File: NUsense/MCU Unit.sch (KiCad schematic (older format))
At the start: 45 parts, among them SW301 SW_Push, U301 STM32F746ZGT6, X301 24MHz, X302 ST3215SB32768H5

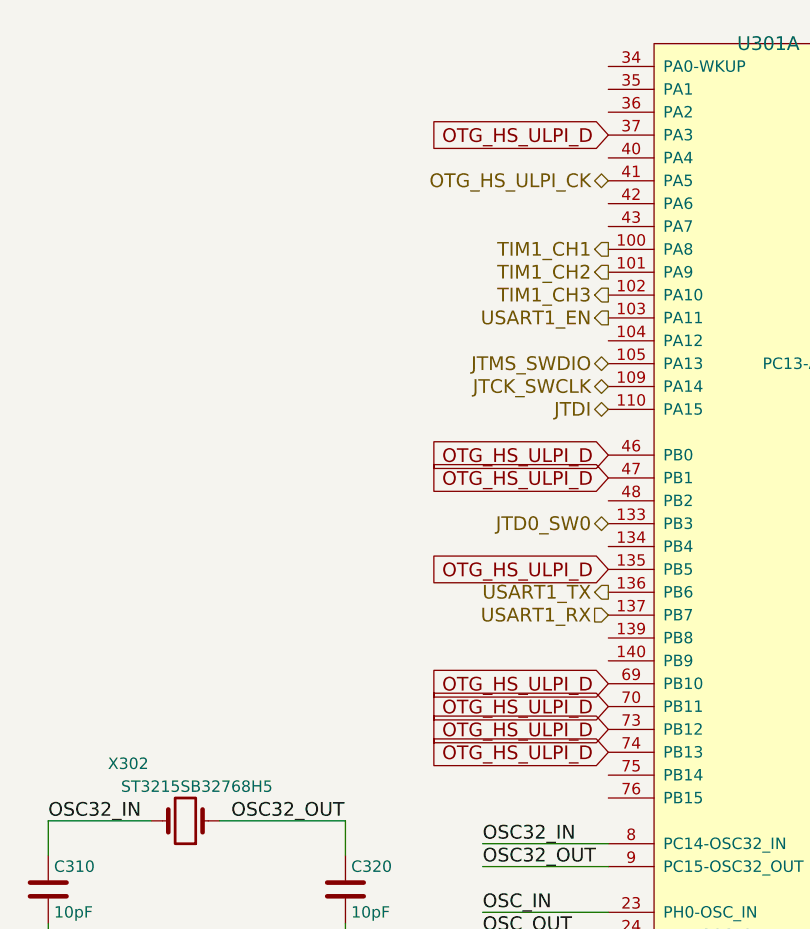
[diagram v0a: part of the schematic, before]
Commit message: Cleans up some minor things
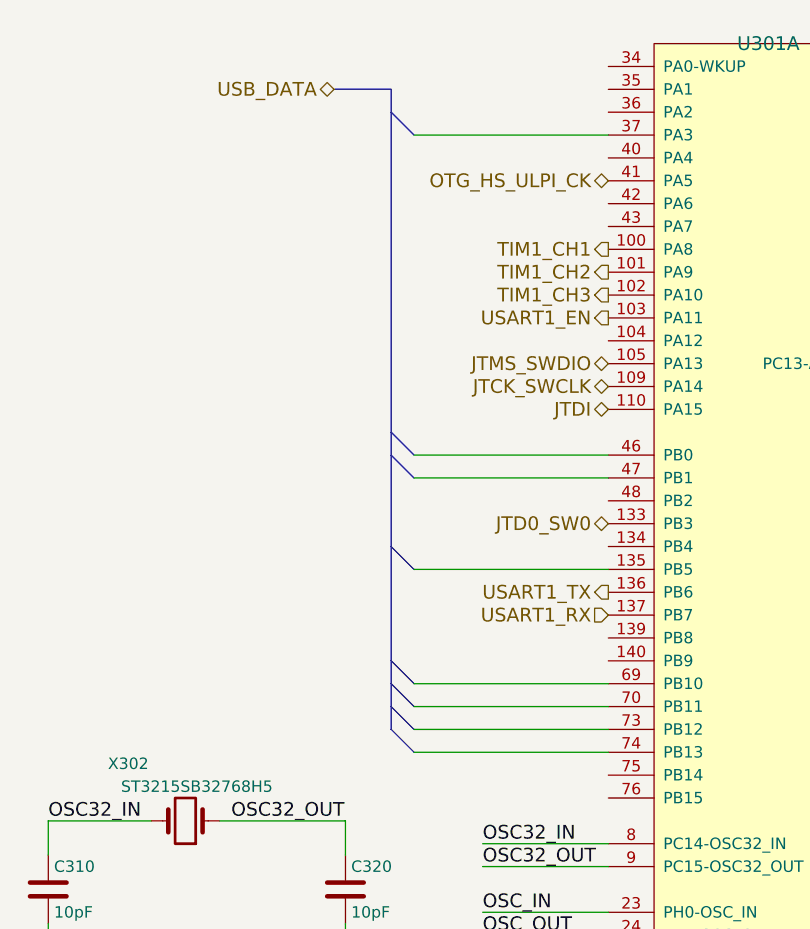
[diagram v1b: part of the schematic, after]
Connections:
- net labels added: USB_DATA
- net labels removed: OTG_HS_ULPI_D
- wire segments 141 -> 149
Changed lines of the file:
@@
 $EndComp
 $Comp
-L GND #PWR14
+L GND #PWR306
 U 1 1 5A6BFE16
 P 4000 6200
-F 0 "#PWR14" H 4000 5950 50  0001 C CNN
+F 0 "#PWR306" H 4000 5950 50  0001 C CNN
 F 1 "GND" H 4000 6050 50  0000 C CNN
 F 2 "" H 4000 6200 50  0001 C CNN
@@
 $EndComp
 $Comp
-L GND #PWR11
+L GND #PWR303
 U 1 1 5A6BFE38
 P 3200 6950
-F 0 "#PWR11" H 3200 6700 50  0001 C CNN
+F 0 "#PWR303" H 3200 6700 50  0001 C CNN
 F 1 "GND" H 3200 6800 50  0000 C CNN
 F 2 "" H 3200 6950 50  0001 C CNN
@@
 $EndComp
 $Comp
-L GND #PWR13
+L GND #PWR305
 U 1 1 5A6BFE45
 P 3800 7150
-F 0 "#PWR13" H 3800 6900 50  0001 C CNN
+F 0 "#PWR305" H 3800 6900 50  0001 C CNN
 F 1 "GND" H 3800 7000 50  0000 C CNN
 F 2 "" H 3800 7150 50  0001 C CNN
@@
 $EndComp
 $Comp
-L GND #PWR9
+L GND #PWR301
 U 1 1 5A6BFE4B
 P 2650 7150
-F 0 "#PWR9" H 2650 6900 50  0001 C CNN
+F 0 "#PWR301" H 2650 6900 50  0001 C CNN
 F 1 "GND" H 2650 7000 50  0000 C CNN
 F 2 "" H 2650 7150 50  0001 C CNN
@@
 $EndComp
 $Comp
-L GND #PWR16
+L GND #PWR308
 U 1 1 5A6BFE84
 P 4950 8100
-F 0 "#PWR16" H 4950 7850 50  0001 C CNN
+F 0 "#PWR308" H 4950 7850 50  0001 C CNN
 F 1 "GND" H 4950 7950 50  0000 C CNN
 F 2 "" H 4950 8100 50  0001 C CNN
@@
 $EndComp
 $Comp
-L GND #PWR21
+L GND #PWR313
 U 1 1 5A6BFE8A
 P 6700 7300
-F 0 "#PWR21" H 6700 7050 50  0001 C CNN
+F 0 "#PWR313" H 6700 7050 50  0001 C CNN
 F 1 "GND" H 6700 7150 50  0000 C CNN
 F 2 "" H 6700 7300 50  0001 C CNN
@@
 $EndComp
 $Comp
-L GND #PWR26
+L GND #PWR318
 U 1 1 5A6BFEA7
 P 8750 9450
-F 0 "#PWR26" H 8750 9200 50  0001 C CNN
+F 0 "#PWR318" H 8750 9200 50  0001 C CNN
 F 1 "GND" H 8750 9300 50  0000 C CNN
 F 2 "" H 8750 9450 50  0001 C CNN
@@
 $EndComp
 $Comp
-L GND #PWR23
+L GND #PWR315
 U 1 1 5A6BFEDA
 P 8050 10650
-F 0 "#PWR23" H 8050 10400 50  0001 C CNN
+F 0 "#PWR315" H 8050 10400 50  0001 C CNN
 F 1 "GND" H 8050 10500 50  0000 C CNN
 F 2 "" H 8050 10650 50  0001 C CNN
@@
 $EndComp
 $Comp
-L GND #PWR25
+L GND #PWR317
 U 1 1 5A6BFEE0
 P 8400 10650
-F 0 "#PWR25" H 8400 10400 50  0001 C CNN
+F 0 "#PWR317" H 8400 10400 50  0001 C CNN
 F 1 "GND" H 8400 10500 50  0000 C CNN
 F 2 "" H 8400 10650 50  0001 C CNN
@@
 $EndComp
 $Comp
-L GND #PWR27
+L GND #PWR319
 U 1 1 5A6BFEE6
 P 8750 10650
-F 0 "#PWR27" H 8750 10400 50  0001 C CNN
+F 0 "#PWR319" H 8750 10400 50  0001 C CNN
 F 1 "GND" H 8750 10500 50  0000 C CNN
 F 2 "" H 8750 10650 50  0001 C CNN
@@
 $EndComp
 $Comp
-L GND #PWR28
+L GND #PWR320
 U 1 1 5A6BFEEC
 P 9050 10650
-F 0 "#PWR28" H 9050 10400 50  0001 C CNN
+F 0 "#PWR320" H 9050 10400 50  0001 C CNN
 F 1 "GND" H 9050 10500 50  0000 C CNN
 F 2 "" H 9050 10650 50  0001 C CNN
@@
 $EndComp
 $Comp
-L GND #PWR29
+L GND #PWR321
 U 1 1 5A6BFEF3
 P 11000 9500
-F 0 "#PWR29" H 11000 9250 50  0001 C CNN
+F 0 "#PWR321" H 11000 9250 50  0001 C CNN
 F 1 "GND" H 11000 9350 50  0000 C CNN
 F 2 "" H 11000 9500 50  0001 C CNN
@@
 $EndComp
 $Comp
-L GND #PWR30
+L GND #PWR322
 U 1 1 5A6BFF00
 P 11000 10500
-F 0 "#PWR30" H 11000 10250 50  0001 C CNN
+F 0 "#PWR322" H 11000 10250 50  0001 C CNN
 F 1 "GND" H 11000 10350 50  0000 C CNN
 F 2 "" H 11000 10500 50  0001 C CNN
@@
 $EndComp
 $Comp
-L GND #PWR31
+L GND #PWR323
 U 1 1 5A6BFF06
 P 11300 10500
-F 0 "#PWR31" H 11300 10250 50  0001 C CNN
+F 0 "#PWR323" H 11300 10250 50  0001 C CNN
 F 1 "GND" H 11300 10350 50  0000 C CNN
 F 2 "" H 11300 10500 50  0001 C CNN
@@
 $EndComp
 $Comp
-L GND #PWR15
+L GND #PWR307
 U 1 1 5A6BFF68
 P 4550 10350
-F 0 "#PWR15" H 4550 10100 50  0001 C CNN
+F 0 "#PWR307" H 4550 10100 50  0001 C CNN
 F 1 "GND" H 4550 10200 50  0000 C CNN
 F 2 "" H 4550 10350 50  0001 C CNN
@@
 Wire Wire Line
 	11300 9900 11300 10100
-Text GLabel 5150 2600 0    60   Input ~ 0
-OTG_HS_ULPI_D
-Text GLabel 5150 4000 0    60   Input ~ 0
-OTG_HS_ULPI_D
-Text GLabel 5150 4100 0    60   Input ~ 0
-OTG_HS_ULPI_D
-Text GLabel 5150 4500 0    60   Input ~ 0
-OTG_HS_ULPI_D
-Text GLabel 5150 5000 0    60   Input ~ 0
-OTG_HS_ULPI_D
-Text GLabel 5150 5100 0    60   Input ~ 0
-OTG_HS_ULPI_D
-Text GLabel 5150 5200 0    60   Input ~ 0
-OTG_HS_ULPI_D
-Text GLabel 5150 5300 0    60   Input ~ 0
-OTG_HS_ULPI_D
-$Comp
-L +3.3V #PWR20
+$Comp
+L +3.3V #PWR312
 U 1 1 5A6FCDF0
 P 6700 7000
-F 0 "#PWR20" H 6700 6850 50  0001 C CNN
+F 0 "#PWR312" H 6700 6850 50  0001 C CNN
 F 1 "+3.3V" H 6700 7140 50  0000 C CNN
 F 2 "" H 6700 7000 50  0001 C CNN
@@
 $EndComp
 $Comp
-L +3.3V #PWR18
+L +3.3V #PWR310
 U 1 1 5A6FCE7A
 P 5800 7500
-F 0 "#PWR18" H 5800 7350 50  0001 C CNN
+F 0 "#PWR310" H 5800 7350 50  0001 C CNN
 F 1 "+3.3V" H 5800 7640 50  0000 C CNN
 F 2 "" H 5800 7500 50  0001 C CNN
@@
 $EndComp
 $Comp
-L +3.3V #PWR24
+L +3.3V #PWR316
 U 1 1 5A6FD2DC
 P 8250 8400
-F 0 "#PWR24" H 8250 8250 50  0001 C CNN
+F 0 "#PWR316" H 8250 8250 50  0001 C CNN
 F 1 "+3.3V" H 8250 8540 50  0000 C CNN
 F 2 "" H 8250 8400 50  0001 C CNN
@@
 VDD3o3V_MCU
 $Comp
-L GND #PWR17
+L GND #PWR309
 U 1 1 5A701246
 P 5500 9800
-F 0 "#PWR17" H 5500 9550 50  0001 C CNN
+F 0 "#PWR309" H 5500 9550 50  0001 C CNN
 F 1 "GND" H 5500 9650 50  0000 C CNN
 F 2 "" H 5500 9800 50  0001 C CNN
@@
 VDD_REF+
 $Comp
-L GND #PWR19
+L GND #PWR311
 U 1 1 5A7014A6
 P 6300 10750
-F 0 "#PWR19" H 6300 10500 50  0001 C CNN
+F 0 "#PWR311" H 6300 10500 50  0001 C CNN
 F 1 "GND" H 6300 10600 50  0000 C CNN
 F 2 "" H 6300 10750 50  0001 C CNN
@@
 	8400 9650 8400 10300
 $Comp
-L +3.3V #PWR22
+L +3.3V #PWR314
 U 1 1 5A6FD08D
 P 6900 9900
-F 0 "#PWR22" H 6900 9750 50  0001 C CNN
+F 0 "#PWR314" H 6900 9750 50  0001 C CNN
 F 1 "+3.3V" H 6900 10040 50  0000 C CNN
 F 2 "" H 6900 9900 50  0001 C CNN
@@
 $EndComp
 $Comp
-L GND #PWR10
+L GND #PWR302
 U 1 1 5A6BFE10
 P 2700 6200
-F 0 "#PWR10" H 2700 5950 50  0001 C CNN
+F 0 "#PWR302" H 2700 5950 50  0001 C CNN
 F 1 "GND" H 2700 6050 50  0000 C CNN
 F 2 "" H 2700 6200 50  0001 C CNN
@@
 	5150 5800 4600 5800
 $Comp
-L GND #PWR12
+L GND #PWR304
 U 1 1 5A7647F9
 P 3400 6450
-F 0 "#PWR12" H 3400 6200 50  0001 C CNN
+F 0 "#PWR304" H 3400 6200 50  0001 C CNN
 F 1 "GND" H 3400 6300 50  0000 C CNN
 F 2 "" H 3400 6450 50  0001 C CNN
@@
 Text HLabel 6650 3100 2    60   Output ~ 0
 TIM8_CH3
+Entry Bus Bus
+	4200 2500 4300 2600
+Entry Bus Bus
+	4200 3900 4300 4000
+Entry Bus Bus
+	4200 4000 4300 4100
+Entry Bus Bus
+	4200 4400 4300 4500
+Entry Bus Bus
+	4200 4900 4300 5000
+Entry Bus Bus
+	4200 5000 4300 5100
+Entry Bus Bus
+	4200 5100 4300 5200
+Entry Bus Bus
+	4200 5200 4300 5300
+Wire Bus Line
+	4200 5200 4200 2400
+Wire Bus Line
+	4200 2400 3950 2400
+Text HLabel 3950 2400 0    60   BiDi ~ 0
+USB_DATA
+Wire Wire Line
+	5150 5300 4300 5300
+Wire Wire Line
+	5150 5200 4300 5200
+Wire Wire Line
+	5150 5100 4300 5100
+Wire Wire Line
+	5150 5000 4300 5000
+Wire Wire Line
+	5150 4500 4300 4500
+Wire Wire Line
+	5150 4100 4300 4100
+Wire Wire Line
+	5150 4000 4300 4000
+Wire Wire Line
+	4300 2600 5150 2600
 $EndSCHEMATC
